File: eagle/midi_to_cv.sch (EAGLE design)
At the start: 57 parts, among them IC1 TL074P, IC2 4504N, IC3 4099N, IC4 TL074P, U1 ATMEGA328P_PDIP

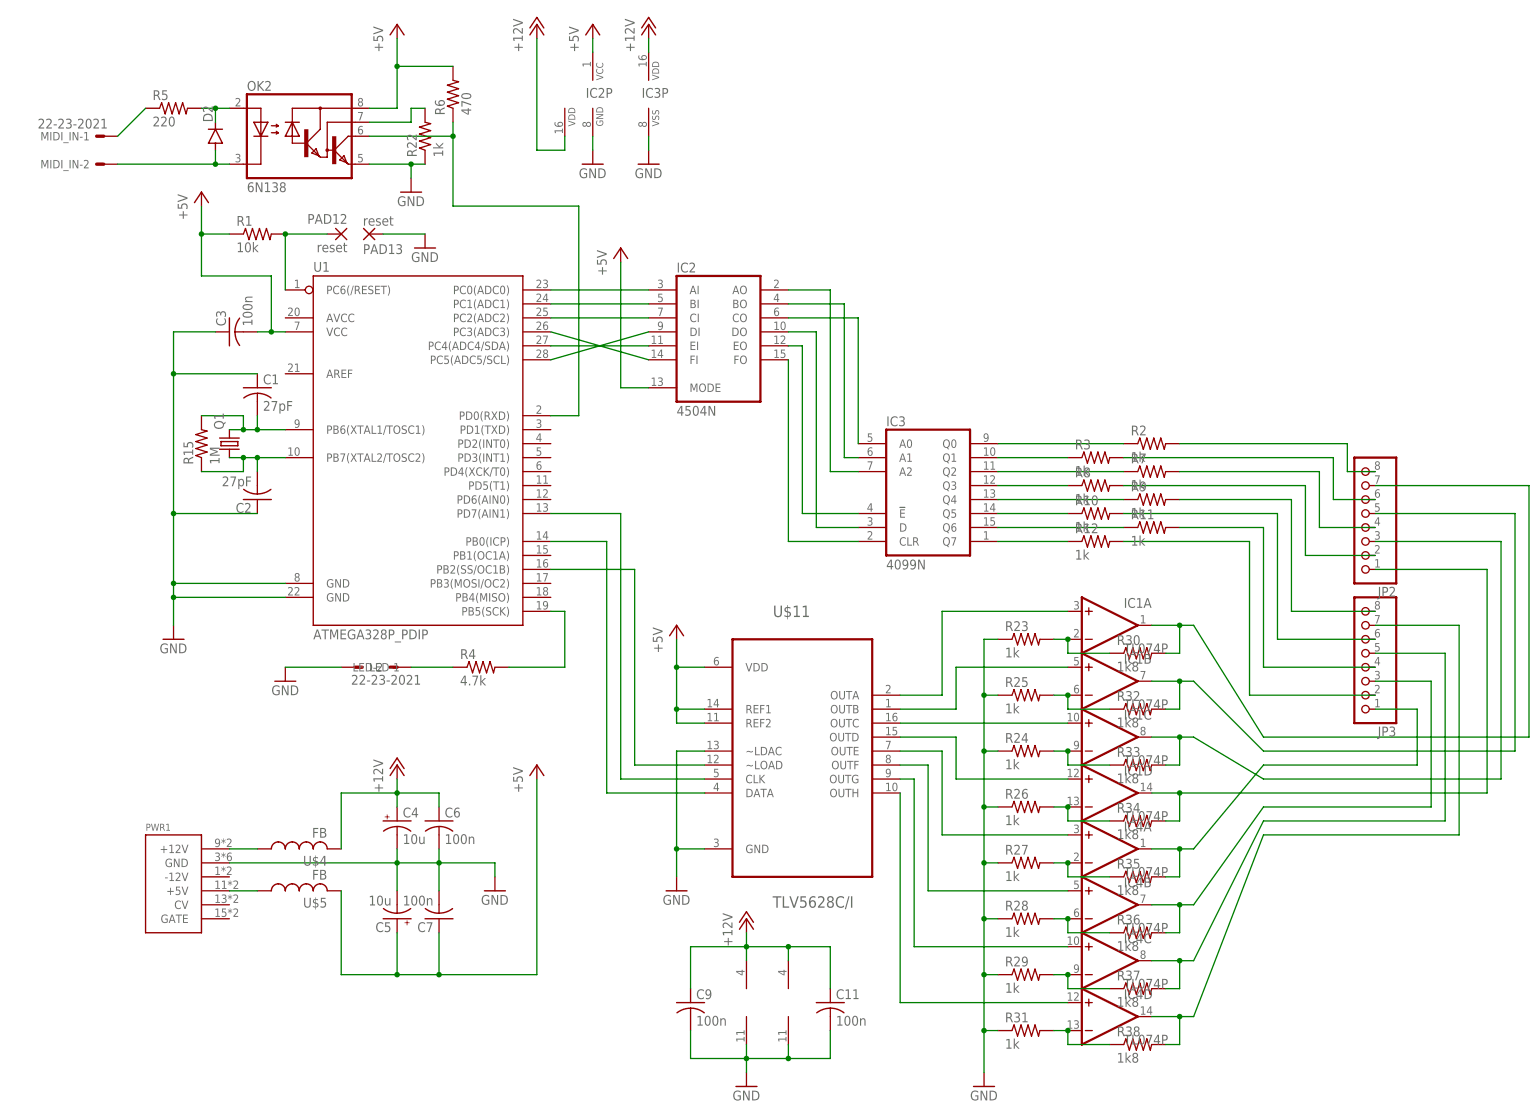
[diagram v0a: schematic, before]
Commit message: reverted to working midi board
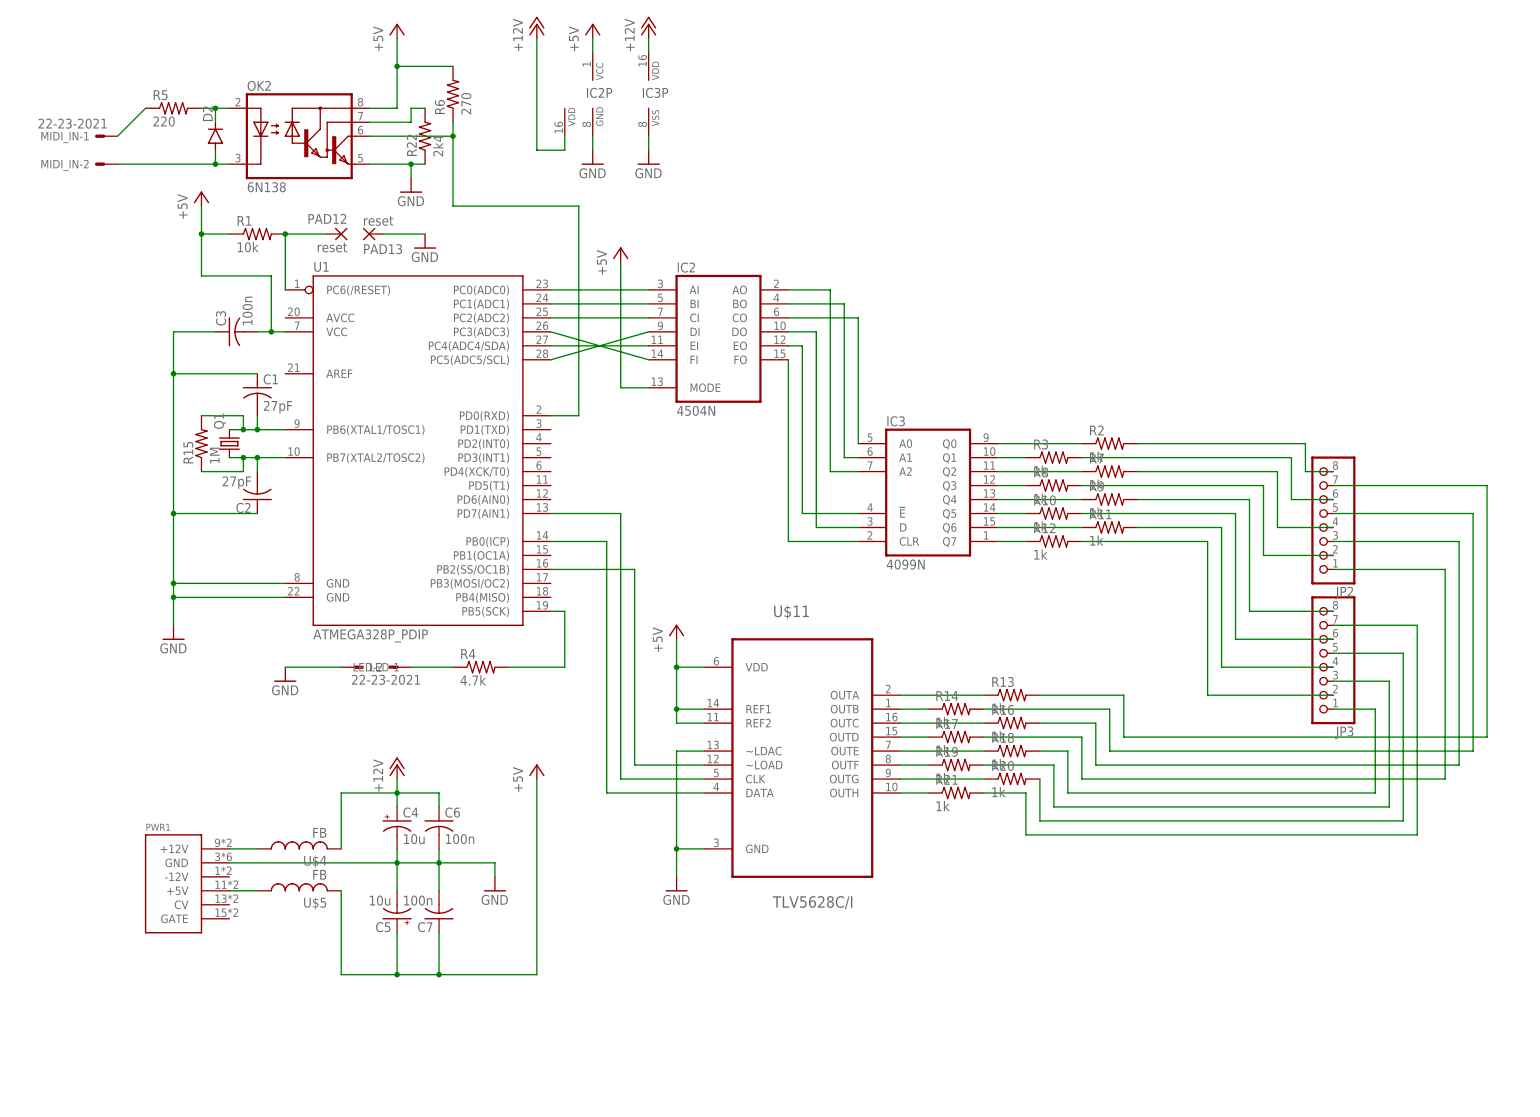
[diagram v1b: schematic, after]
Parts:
- removed C11, C9: 100n, rcl:C-US050-024X044
- removed IC1, IC4: TL074P, linear:TL074P
- removed R23, R24, R25, R26, R27, R28, R29, R31: 1k, rcl:R-US_0207/10
- removed R30, R32, R33, R34, R35, R36, R37, R38: 1k8, rcl:R-US_0204/2V
- added R13, R14, R16, R17, R18, R19, R20, R21: 1k, rcl:R-US_0207/10
- R22: value 1k -> 2k4
- R6: value 470 -> 270
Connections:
- removed net N$43: IC4D.+IN, U$11.OUTH
- removed net N$63: IC1D.-IN, R26.2, R34.1
- removed net N$64: IC4A.-IN, R27.2, R35.1
- removed net N$65: IC4B.-IN, R28.2, R36.1
- removed net N$66: IC4C.-IN, R29.2, R37.1
- removed net N$67: IC4D.-IN, R31.2, R38.1
- removed net N$68: IC1D.+IN, U$11.OUTD
- removed net N$69: IC1C.+IN, U$11.OUTC
- removed net N$70: IC1B.+IN, U$11.OUTB
- removed net N$71: IC1A.+IN, U$11.OUTA
- new net N$24: JP2.5, R14.2
- new net N$40: JP3.1, R18.2
- net +12V: no longer C11.1, C9.1, IC1P.V+, IC4P.V+
- net GND: no longer C11.2, C9.2, IC1P.V-, IC4P.V-, R23.1, R24.1, R25.1, R26.1, R27.1, R28.1, R29.1, R31.1
- net N$22: now also R13.2; no longer IC1A.OUT, R30.2
- net N$28: now also R16.2; no longer IC1C.OUT, R33.2
- net N$29: now also R17.2; no longer IC1D.OUT, R34.2
- net N$34: now also R20.2; no longer IC4C.OUT, R37.2
- net N$41: now also R19.2; no longer IC4B.OUT, R36.2
- net N$51: now also R21.2; no longer IC4D.OUT, R38.2
- net N$52: now also R13.1, U$11.OUTA; no longer IC4A.OUT, JP3.1, R35.2
- net N$53: now also R14.1, U$11.OUTB; no longer IC4C.+IN, U$11.OUTG
- net N$54: now also R16.1, U$11.OUTC; no longer IC4B.+IN, U$11.OUTF
- net N$55: now also R17.1, U$11.OUTD; no longer IC4A.+IN, U$11.OUTE
- net N$56: now also R18.1, U$11.OUTE; no longer IC1B.OUT, JP2.5, R32.2
- net N$57: now also R19.1, U$11.OUTF; no longer IC1A.-IN, R23.2, R30.1
- net N$58: now also R20.1, U$11.OUTG; no longer IC1C.-IN, R24.2, R33.1
- net N$59: now also R21.1, U$11.OUTH; no longer IC1B.-IN, R25.2, R32.1
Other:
- moved on the sheet: JP2, JP3, R10, R11, R12, R2, R3, R7, R8, R9
